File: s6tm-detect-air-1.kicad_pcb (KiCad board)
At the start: 2 copper layers, 67 x 67 mm, 82 parts, among them J1 Conn_01x04, J2 TC2030, J3 Conn_01x04, J4 Conn_01x04, J5 Conn_01x04_Pin, J6 Conn_01x08, SW1 SW_Push, SW2 SW_Push, U1 SYS1002-H2, U10 004-1-0100, U2 MiCS-5524, U3 LMC6482, U4 HT753-1, U5 SN65HVD230, U6 STM32F103C8Tx, U7 HTU21, U8 LM73100, U9 ENS16x, Y1 8M

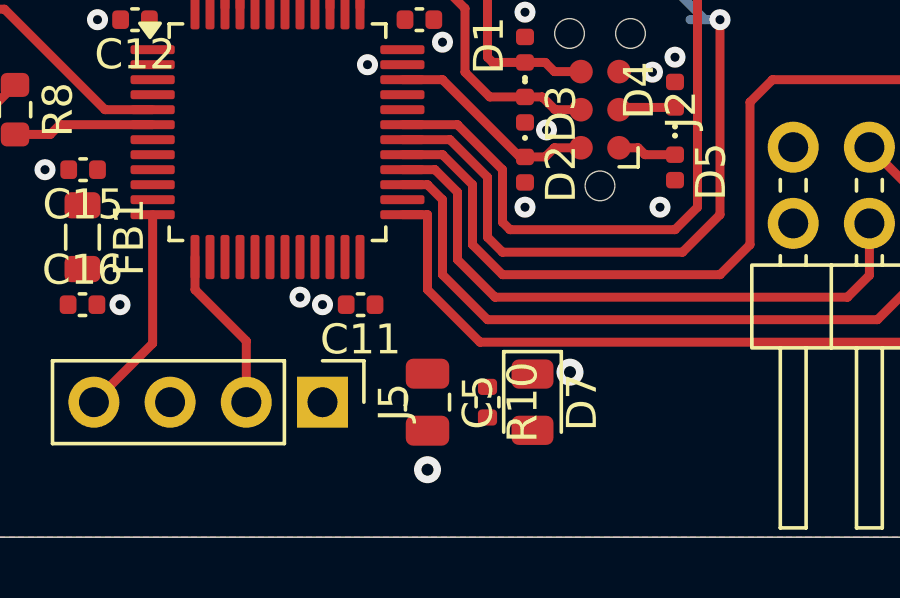
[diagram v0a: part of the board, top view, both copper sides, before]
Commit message: pcb: add status led routing
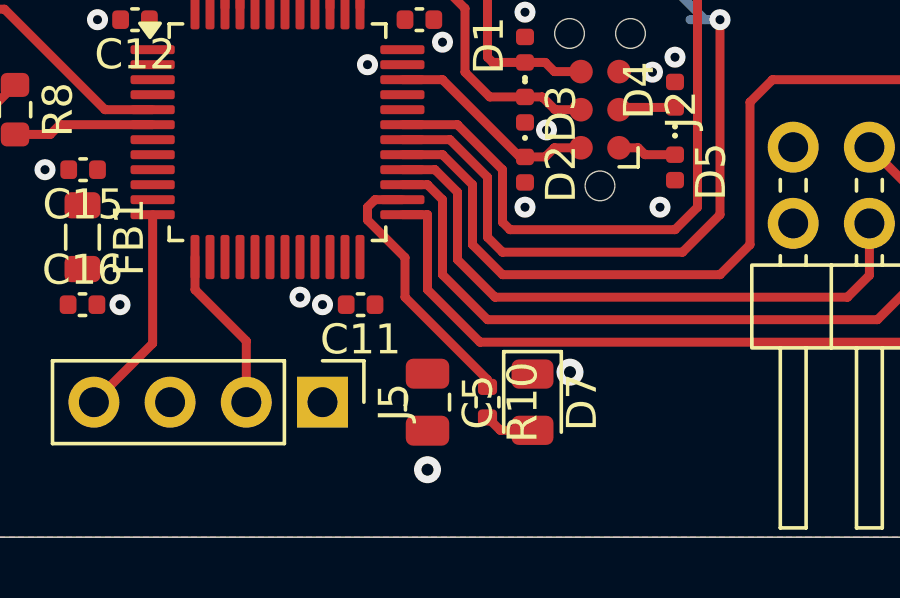
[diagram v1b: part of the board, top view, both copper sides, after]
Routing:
- net Net-(U6-PB13): track 0.00 -> 8.91 mm
- net Net-(D7-A): track 0.00 -> 1.68 mm
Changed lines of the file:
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@@
+	)
+	(segment
+		(start 144.4275 116.4375)
+		(end 145.5 116.4375)
+		(width 0.3)
+		(layer "F.Cu")
+		(net "Net-(D7-A)")
+	)
+	(segment
+		(start 144 116.01)
+		(end 144.4275 116.4375)
+		(width 0.3)
+		(layer "F.Cu")
+		(net "Net-(D7-A)")
 	)
 	(segment
@@
 		(net "/PB14")
 	)
+	(segment
+		(start 144 114.99)
+		(end 144 114.75)
+		(width 0.3)
+		(layer "F.Cu")
+		(net "Net-(U6-PB13)")
+	)
+	(segment
+		(start 144 114.75)
+		(end 141.25 112)
+		(width 0.3)
+		(layer "F.Cu")
+		(net "Net-(U6-PB13)")
+	)
+	(segment
+		(start 140.25 108.75)
+		(end 141.1625 108.75)
+		(width 0.3)
+		(layer "F.Cu")
+		(net "Net-(U6-PB13)")
+	)
+	(segment
+		(start 141.25 110.678705)
+		(end 140 109.428705)
+		(width 0.3)
+		(layer "F.Cu")
+		(net "Net-(U6-PB13)")
+	)
+	(segment
+		(start 140 109.428705)
+		(end 140 109)
+		(width 0.3)
+		(layer "F.Cu")
+		(net "Net-(U6-PB13)")
+	)
+	(segment
+		(start 141.25 112)
+		(end 141.25 110.678705)
+		(width 0.3)
+		(layer "F.Cu")
+		(net "Net-(U6-PB13)")
+	)
+	(segment
+		(start 140 109)
+		(end 140.25 108.75)
+		(width 0.3)
+		(layer "F.Cu")
+		(net "Net-(U6-PB13)")
+	)
 	(zone
